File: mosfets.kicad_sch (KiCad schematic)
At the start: 32 parts, among them IC6 KTS1622EUAA-TR, J2 Screw_Terminal_01x02, J3 Screw_Terminal_01x02, J4 Screw_Terminal_01x02, J5 Screw_Terminal_01x02, J6 Screw_Terminal_01x02, J7 Screw_Terminal_01x02, Q1 IRLML6402, Q10 IRLML6244, Q11 IRLML6402, Q12 IRLML6244, Q2 IRLML6244, Q3 IRLML6402, Q4 IRLML6244, Q5 IRLML6402, Q6 IRLML6244, Q7 IRLML6402, Q8 IRLML6244, Q9 IRLML6402

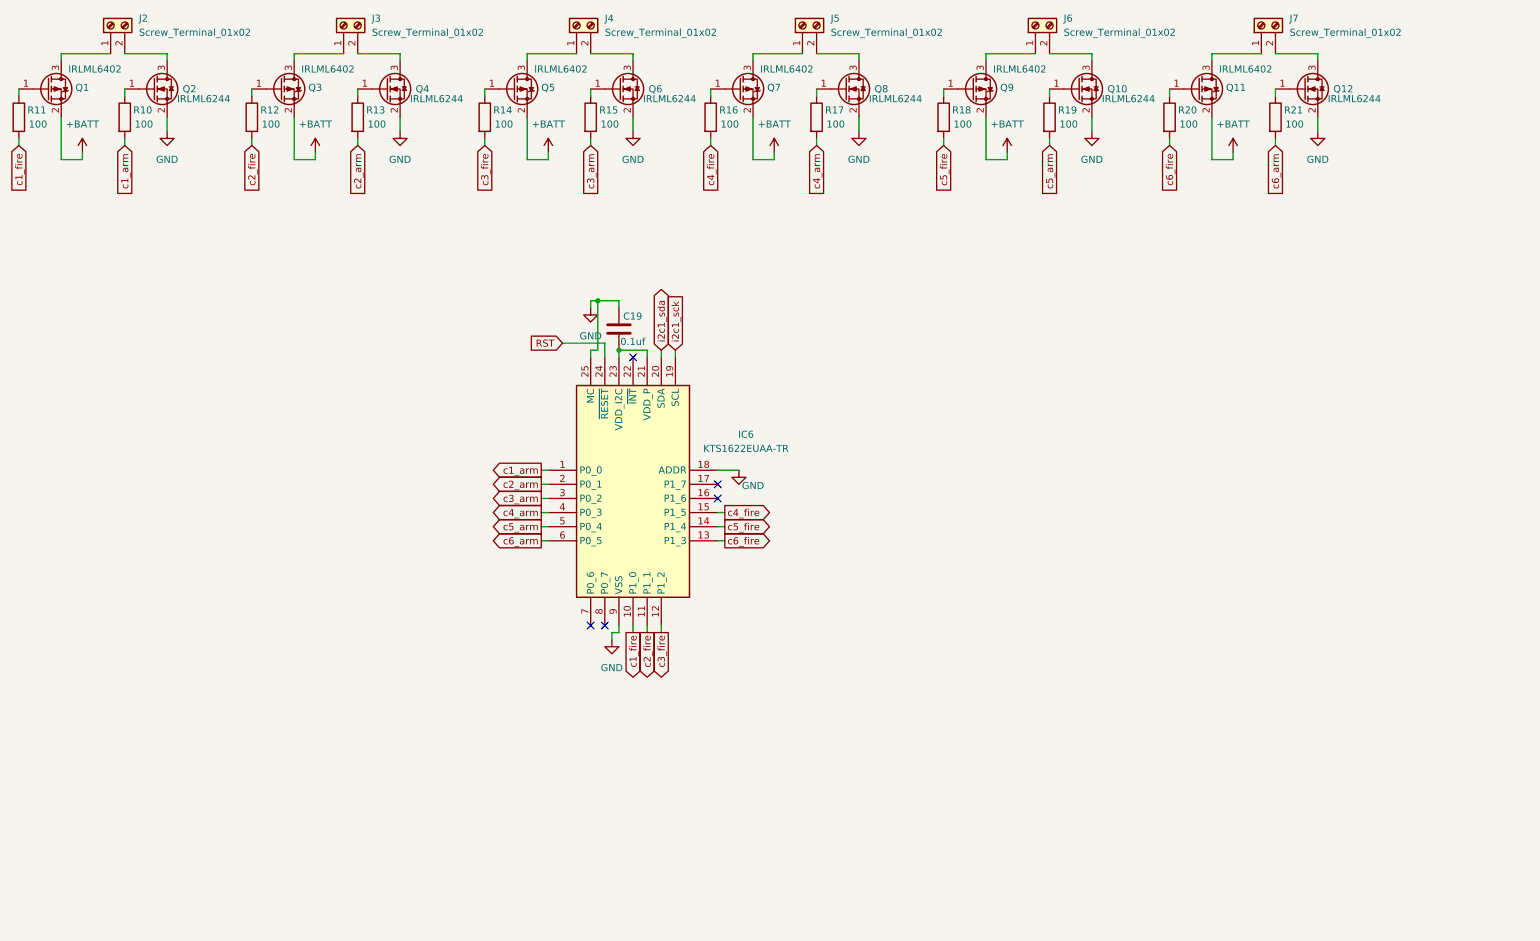
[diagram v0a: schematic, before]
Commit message: pcb coming along, schematic way more done - I now have a lot more respect for hardware people than I did earlier
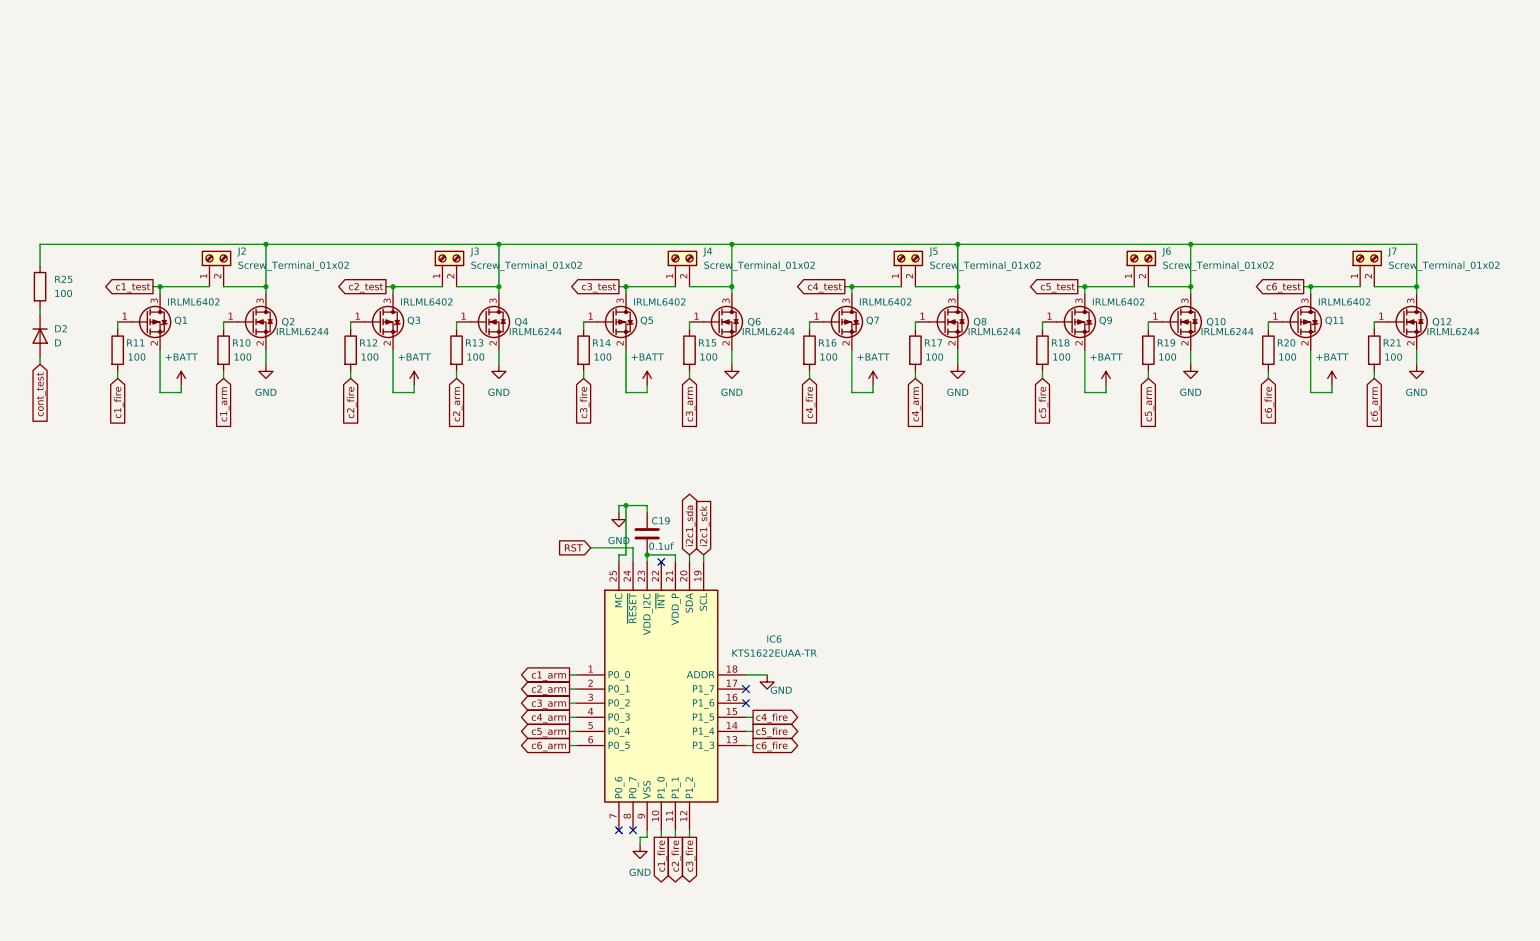
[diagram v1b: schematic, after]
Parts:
- added D2: D, Diode_SMD:D_0402_1005Metric, symbol Device:D
- added R25: 100, Resistor_SMD:R_0805_2012Metric, symbol Device:R
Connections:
- net c2_test: now reaches J3.1 (Pin_1), Q3.3 (D)
- net at J3.2 (Pin_2), Q4.3 (D): now also J2.2 (Pin_2), J4.2 (Pin_2), J5.2 (Pin_2), J6.2 (Pin_2), J7.2 (Pin_2), Q10.3 (D), Q12.3 (D), Q2.3 (D), Q6.3 (D), Q8.3 (D), R25.1
- net c4_test: now reaches J5.1 (Pin_1), Q7.3 (D)
- net c3_test: now reaches J4.1 (Pin_1), Q5.3 (D)
- net c6_test: now reaches J7.1 (Pin_1), Q11.3 (D)
- net c1_test: now reaches J2.1 (Pin_1), Q1.3 (D)
- net c5_test: now reaches J6.1 (Pin_1), Q9.3 (D)
- new net: D2.1 (K), R25.2
- new net cont_test: D2.2 (A)
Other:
- moved on the sheet: C19, IC6, J2, J3, J4, J5, J6, J7, Q1, Q10, Q11, Q12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

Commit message: tons of work, see journal for details
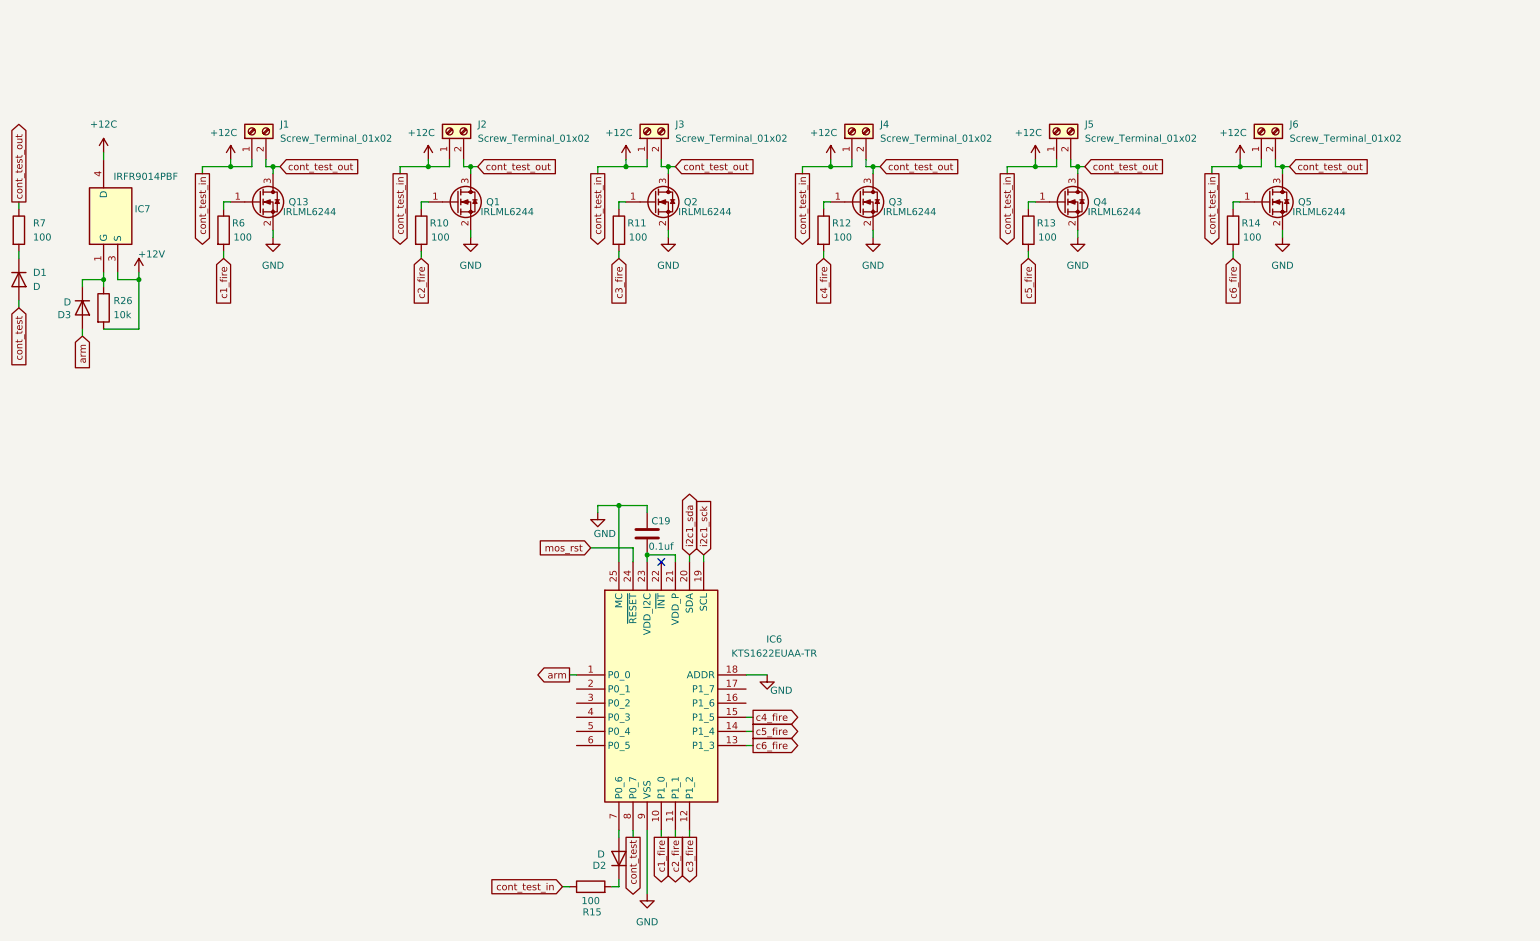
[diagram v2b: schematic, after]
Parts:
- removed J7: Screw_Terminal_01x02, symbol Connector:Screw_Terminal_01x02
- removed Q1, Q11, Q3, Q5, Q7, Q9: IRLML6402, Package_TO_SOT_SMD:SOT-23, symbol Transistor_FET:IRLML6402
- removed Q10, Q12, Q6, Q8: IRLML6244, Package_TO_SOT_SMD:SOT-23, symbol Transistor_FET:IRLML6244
- removed R16, R17, R18, R19, R20, R21: 100, Resistor_SMD:R_0201_0603Metric, symbol Device:R
- removed R25: 100, Resistor_SMD:R_0805_2012Metric, symbol Device:R
- added D1: D, Diode_SMD:D_0402_1005Metric, symbol Device:D
- added D3: D, symbol Device:D
- added IC7: IRFR9014PBF, TO228P990X238-3N, symbol IRFR9014PBF:IRFR9014PBF
- added J1: Screw_Terminal_01x02, symbol Connector:Screw_Terminal_01x02
- added Q1, Q13, Q3, Q5: IRLML6244, Package_TO_SOT_SMD:SOT-23, symbol Transistor_FET:IRLML6244
- added R26: 10k, symbol Device:R
- added R6: 100, Resistor_SMD:R_0201_0603Metric, symbol Device:R
- added R7: 100, Resistor_SMD:R_0805_2012Metric, symbol Device:R
- D2: footprint Diode_SMD:D_0402_1005Metric -> (none)
- R15: footprint Resistor_SMD:R_0201_0603Metric -> (none)
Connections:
- net c1_test is gone; now on net +12C: J2.1 (Pin_1)
- net c2_test is gone; now on net +12C: J3.1 (Pin_1)
- net c3_test is gone; now on net +12C: J4.1 (Pin_1)
- net c4_test is gone; now on net +12C: J5.1 (Pin_1)
- net c5_test is gone; now on net +12C: J6.1 (Pin_1)
- net GND: now also Q1.2 (S), Q13.2 (S), Q3.2 (S), Q5.2 (S)
- net c1_fire: now also R6.2; no longer R11.2
- net c2_fire: now also R10.2; no longer R12.2
- net c3_fire: now also R11.2; no longer R14.2
- net c4_fire: now also R12.2
- net c5_fire: now also R13.2
- net c6_fire: now also R14.2
- net cont_test: now also IC6.8 (P0_7), D1.2 (A); no longer D2.2 (A)
- net cont_test_out: now reaches J2.2 (Pin_2), J3.2 (Pin_2), J4.2 (Pin_2), J5.2 (Pin_2), J6.2 (Pin_2), Q2.3 (D), Q4.3 (D)
- net cont_test_out: now also J1.2 (Pin_2), Q1.3 (D), Q13.3 (D), Q3.3 (D), Q5.3 (D), R7.1
- net at D2.1 (K): now also R15.2
- net at R12.1: now also Q3.1 (G)
- net +12C: now reaches R15.1
- net +12C: now also IC7.4 (D), J1.1 (Pin_1)
- net at R11.1: now also Q2.1 (G)
- net at R10.1: now also Q1.1 (G); no longer Q2.1 (G)
- net at IC6.7 (P0_6): now also D2.2 (A)
- net at R14.1: now also Q5.1 (G)
- net RST renamed mos_rst
- net c1_arm renamed arm
- net arm: now also D3.2 (A); no longer R10.2
- net c2_arm: no longer names the net of IC6.2 (P0_1)
- net c2_arm: no longer R13.2
- net c3_arm: no longer names the net of IC6.3 (P0_2)
- net c3_arm: no longer R15.2
- net c4_arm: no longer names the net of IC6.4 (P0_3)
- net c5_arm: no longer names the net of IC6.5 (P0_4)
- net c6_arm: no longer names the net of IC6.6 (P0_5)
- new net: D3.1 (K), IC7.1 (G), R26.1
- new net: Q13.1 (G), R6.1
- new net: D1.1 (K), R7.2
- new net +12V: IC7.3 (S), R26.2
- no-connect marks 5 -> 1
